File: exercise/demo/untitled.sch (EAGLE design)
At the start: 9 parts, among them Q1 S8050SOT23

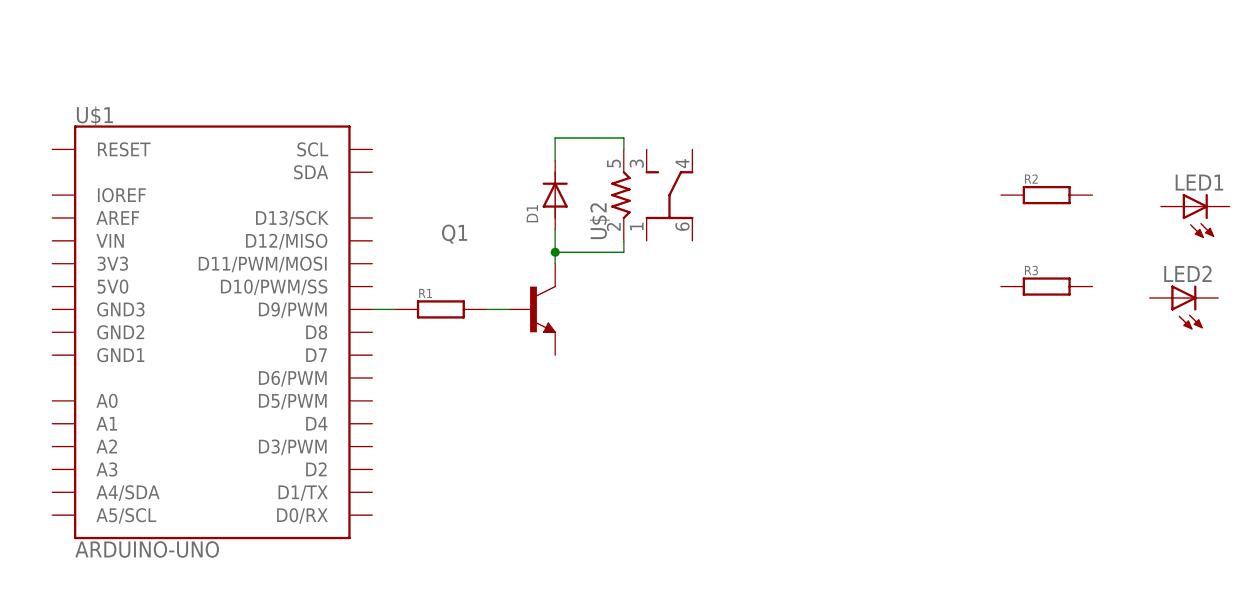
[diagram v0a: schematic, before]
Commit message: 2020.07.08.01
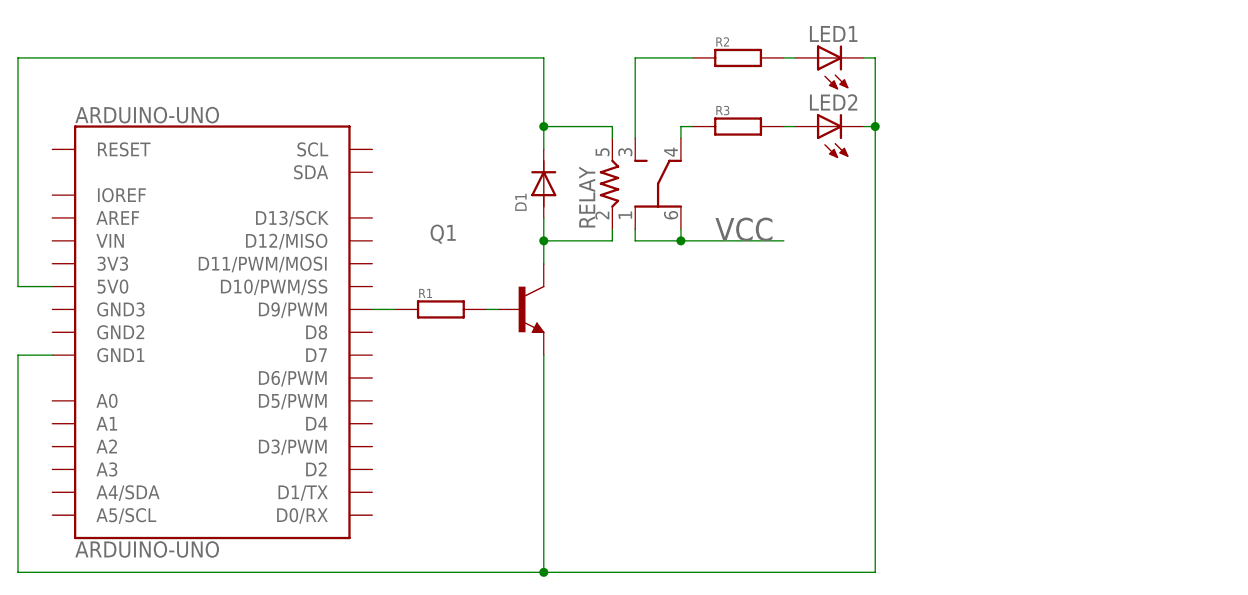
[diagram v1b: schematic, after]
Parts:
- removed U$2: RELAY-HK4100F-DC5V, Senser:RELAY-HK4100F-DC5V
- added RELAY: RELAY-HK4100F-DC5V, Senser:RELAY-HK4100F-DC5V
- renumbered U$1 to ARDUINO-UNO
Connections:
- new net 5V0: ARDUINO-UNO.5V0, D1.1, RELAY.5
- new net GND: ARDUINO-UNO.GND1, LED1.C, LED2.C, Q1.E
- new net N$11: R2.1, RELAY.3
- new net N$2: LED2.A, R3.2
- new net N$5: R3.1, RELAY.4
- new net VCC: RELAY.1, RELAY.6
- net N$3: now also RELAY.2; no longer U$2.2
- net N$4: now also LED1.A, R2.2; no longer D1.1, U$2.5
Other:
- moved on the sheet: D1, LED1, LED2, Q1, R2, R3
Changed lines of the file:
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@@
 <parts>
 <part name="FRAME1" library="Frame" deviceset="A4-H" device=""/>
-<part name="U$1" library="Module" deviceset="ARDUINO-UNO" device=""/>
-<part name="U$2" library="Senser" deviceset="RELAY-HK4100F-DC5V" device="" value=""/>
+<part name="ARDUINO-UNO" library="Module" deviceset="ARDUINO-UNO" device=""/>
+<part name="RELAY" library="Senser" deviceset="RELAY-HK4100F-DC5V" device="" value=""/>
 <part name="D1" library="RCLDA" deviceset="1N4007" device="SMB" value=""/>
 <part name="Q1" library="RCLDA" deviceset="S8050" device="SOT23" value=""/>
@@
 <instances>
 <instance part="FRAME1" gate="G$1" x="0" y="0"/>
-<instance part="U$1" gate="G$1" x="66.04" y="121.92"/>
-<instance part="U$2" gate="G$1" x="115.57" y="137.16" rot="R90"/>
-<instance part="D1" gate="G$1" x="104.14" y="137.16" rot="R90"/>
-<instance part="Q1" gate="G$1" x="101.6" y="124.46"/>
+<instance part="ARDUINO-UNO" gate="G$1" x="66.04" y="121.92"/>
+<instance part="RELAY" gate="G$1" x="114.3" y="138.43" rot="R90"/>
+<instance part="D1" gate="G$1" x="102.87" y="138.43" rot="R90"/>
+<instance part="Q1" gate="G$1" x="100.33" y="124.46"/>
 <instance part="R1" gate="G$1" x="91.44" y="124.46"/>
-<instance part="R2" gate="G$1" x="158.75" y="137.16"/>
-<instance part="R3" gate="G$1" x="158.75" y="127"/>
-<instance part="LED1" gate="G$1" x="173.99" y="135.89" rot="R90"/>
-<instance part="LED2" gate="G$1" x="172.72" y="125.73" rot="R90"/>
+<instance part="R2" gate="G$1" x="124.46" y="152.4"/>
+<instance part="R3" gate="G$1" x="124.46" y="144.78"/>
+<instance part="LED1" gate="G$1" x="133.35" y="152.4" rot="R90"/>
+<instance part="LED2" gate="G$1" x="133.35" y="144.78" rot="R90"/>
 </instances>
 <busses>
 </busses>
 <nets>
-<net name="N$1" class="0">
+<net name="5V0" class="0">
 <segment>
-<pinref part="U$1" gate="G$1" pin="D9/PWM"/>
+<pinref part="ARDUINO-UNO" gate="G$1" pin="5V0"/>
+<wire x1="48.26" y1="127" x2="44.45" y2="127" width="0.1524" layer="91"/>
+<wire x1="44.45" y1="127" x2="44.45" y2="152.4" width="0.1524" layer="91"/>
+<wire x1="110.49" y1="144.78" x2="102.87" y2="144.78" width="0.1524" layer="91"/>
+<pinref part="RELAY" gate="G$1" pin="5"/>
+<wire x1="110.49" y1="143.51" x2="110.49" y2="144.78" width="0.1524" layer="91"/>
+<wire x1="102.87" y1="144.78" x2="102.87" y2="152.4" width="0.1524" layer="91"/>
+<wire x1="102.87" y1="152.4" x2="44.45" y2="152.4" width="0.1524" layer="91"/>
+<pinref part="D1" gate="G$1" pin="1"/>
+<wire x1="102.87" y1="142.24" x2="102.87" y2="144.78" width="0.1524" layer="91"/>
+<junction x="102.87" y="144.78"/>
+</segment>
+</net>
+<net name="GND" class="0">
+<segment>
+<wire x1="44.45" y1="95.25" x2="44.45" y2="119.38" width="0.1524" layer="91"/>
+<pinref part="ARDUINO-UNO" gate="G$1" pin="GND1"/>
+<wire x1="44.45" y1="119.38" x2="48.26" y2="119.38" width="0.1524" layer="91"/>
+<pinref part="LED1" gate="G$1" pin="C"/>
+<wire x1="138.43" y1="152.4" x2="139.7" y2="152.4" width="0.1524" layer="91"/>
+<wire x1="139.7" y1="152.4" x2="139.7" y2="144.78" width="0.1524" layer="91"/>
+<pinref part="LED2" gate="G$1" pin="C"/>
+<wire x1="139.7" y1="144.78" x2="138.43" y2="144.78" width="0.1524" layer="91"/>
+<wire x1="44.45" y1="95.25" x2="102.87" y2="95.25" width="0.1524" layer="91"/>
+<wire x1="102.87" y1="95.25" x2="139.7" y2="95.25" width="0.1524" layer="91"/>
+<wire x1="139.7" y1="95.25" x2="139.7" y2="144.78" width="0.1524" layer="91"/>
+<junction x="139.7" y="144.78"/>
+<pinref part="Q1" gate="G$1" pin="E"/>
+<wire x1="102.87" y1="119.38" x2="102.87" y2="95.25" width="0.1524" layer="91"/>
+<junction x="102.87" y="95.25"/>
+</segment>
+</net>
+<net name="N$3" class="0">
+<segment>
+<pinref part="RELAY" gate="G$1" pin="2"/>
+<wire x1="110.49" y1="132.08" x2="110.49" y2="133.35" width="0.1524" layer="91"/>
+<wire x1="110.49" y1="132.08" x2="102.87" y2="132.08" width="0.1524" layer="91"/>
+<pinref part="Q1" gate="G$1" pin="C"/>
+<wire x1="102.87" y1="129.54" x2="102.87" y2="132.08" width="0.1524" layer="91"/>
+<pinref part="D1" gate="G$1" pin="2"/>
+<wire x1="102.87" y1="132.08" x2="102.87" y2="134.62" width="0.1524" layer="91"/>
+<junction x="102.87" y="132.08"/>
+</segment>
+</net>
+<net name="N$2" class="0">
+<segment>
+<pinref part="R3" gate="G$1" pin="2"/>
+<pinref part="LED2" gate="G$1" pin="A"/>
+<wire x1="130.81" y1="144.78" x2="129.54" y2="144.78" width="0.1524" layer="91"/>
+</segment>
+</net>
+<net name="N$4" class="0">
+<segment>
+<pinref part="R2" gate="G$1" pin="2"/>
+<pinref part="LED1" gate="G$1" pin="A"/>
+<wire x1="130.81" y1="152.4" x2="129.54" y2="152.4" width="0.1524" layer="91"/>
+</segment>
+</net>
+<net name="N$5" class="0">
+<segment>
+<pinref part="RELAY" gate="G$1" pin="4"/>
+<wire x1="118.11" y1="143.51" x2="118.11" y2="144.78" width="0.1524" layer="91"/>
+<pinref part="R3" gate="G$1" pin="1"/>
+<wire x1="118.11" y1="144.78" x2="119.38" y2="144.78" width="0.1524" layer="91"/>
+</segment>
+</net>
+<net name="N$7" class="0">
+<segment>
+<pinref part="ARDUINO-UNO" gate="G$1" pin="D9/PWM"/>
 <pinref part="R1" gate="G$1" pin="1"/>
 <wire x1="86.36" y1="124.46" x2="83.82" y2="124.46" width="0.1524" layer="91"/>
 </segment>
 </net>
-<net name="N$2" class="0">
+<net name="N$9" class="0">
 <segment>
 <pinref part="R1" gate="G$1" pin="2"/>
 <pinref part="Q1" gate="G$1" pin="B"/>
-<wire x1="99.06" y1="124.46" x2="96.52" y2="124.46" width="0.1524" layer="91"/>
+<wire x1="97.79" y1="124.46" x2="96.52" y2="124.46" width="0.1524" layer="91"/>
 </segment>
 </net>
-<net name="N$3" class="0">
+<net name="N$11" class="0">
 <segment>
-<pinref part="Q1" gate="G$1" pin="C"/>
-<pinref part="D1" gate="G$1" pin="2"/>
-<wire x1="104.14" y1="133.35" x2="104.14" y2="130.81" width="0.1524" layer="91"/>
-<wire x1="104.14" y1="130.81" x2="104.14" y2="129.54" width="0.1524" layer="91"/>
-<wire x1="104.14" y1="130.81" x2="111.76" y2="130.81" width="0.1524" layer="91"/>
-<junction x="104.14" y="130.81"/>
-<pinref part="U$2" gate="G$1" pin="2"/>
-<wire x1="111.76" y1="130.81" x2="111.76" y2="132.08" width="0.1524" layer="91"/>
+<pinref part="R2" gate="G$1" pin="1"/>
+<pinref part="RELAY" gate="G$1" pin="3"/>
+<wire x1="113.03" y1="143.51" x2="113.03" y2="152.4" width="0.1524" layer="91"/>
+<wire x1="113.03" y1="152.4" x2="119.38" y2="152.4" width="0.1524" layer="91"/>
 </segment>
 </net>
-<net name="N$4" class="0">
+<net name="VCC" class="0">
 <segment>
-<pinref part="D1" gate="G$1" pin="1"/>
-<wire x1="104.14" y1="140.97" x2="104.14" y2="143.51" width="0.1524" layer="91"/>
-<wire x1="104.14" y1="143.51" x2="111.76" y2="143.51" width="0.1524" layer="91"/>
-<pinref part="U$2" gate="G$1" pin="5"/>
-<wire x1="111.76" y1="143.51" x2="111.76" y2="142.24" width="0.1524" layer="91"/>
+<pinref part="RELAY" gate="G$1" pin="1"/>
+<pinref part="RELAY" gate="G$1" pin="6"/>
+<wire x1="118.11" y1="133.35" x2="118.11" y2="132.08" width="0.1524" layer="91"/>
+<wire x1="118.11" y1="132.08" x2="113.03" y2="132.08" width="0.1524" layer="91"/>
+<wire x1="113.03" y1="132.08" x2="113.03" y2="133.35" width="0.1524" layer="91"/>
+<wire x1="118.11" y1="132.08" x2="129.54" y2="132.08" width="0.1524" layer="91"/>
+<junction x="118.11" y="132.08"/>
+<label x="121.92" y="132.08" size="2.54" layer="95"/>
 </segment>
 </net>
